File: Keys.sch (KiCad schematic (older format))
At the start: 24 parts

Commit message: experiment
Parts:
- SW? (x10): symbol Keys-rescue:SWITCH_PUSH-Keys-rescue-chgray-keyboard-rescue-chgray-keyboard-rescue -> Cherry-Symbols:SWITCH_PUSH
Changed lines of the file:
@@
 $EndDescr
 $Comp
-L Keys-rescue:SWITCH_PUSH-Keys-rescue-chgray-keyboard-rescue-chgray-keyboard-rescue SW?
+L Cherry-Symbols:SWITCH_PUSH SW?
 U 1 1 58964642
 P 2300 1600
@@
 KEY_ROW0
 $Comp
-L Keys-rescue:SWITCH_PUSH-Keys-rescue-chgray-keyboard-rescue-chgray-keyboard-rescue SW?
+L Cherry-Symbols:SWITCH_PUSH SW?
 U 1 1 589655C0
 P 3050 1600
@@
 $EndComp
 $Comp
-L Keys-rescue:SWITCH_PUSH-Keys-rescue-chgray-keyboard-rescue-chgray-keyboard-rescue SW?
+L Cherry-Symbols:SWITCH_PUSH SW?
 U 1 1 58965EBD
 P 2300 2300
@@
 	2700 1900 2700 2600
 $Comp
-L Keys-rescue:SWITCH_PUSH-Keys-rescue-chgray-keyboard-rescue-chgray-keyboard-rescue SW?
+L Cherry-Symbols:SWITCH_PUSH SW?
 U 1 1 603DF303
 P 3050 2300
@@
 	1800 2600 1800 3550
 $Comp
-L Keys-rescue:SWITCH_PUSH-Keys-rescue-chgray-keyboard-rescue-chgray-keyboard-rescue SW?
+L Cherry-Symbols:SWITCH_PUSH SW?
 U 1 1 603E8C3D
 P 2250 3250
@@
 	1800 3550 1800 4500
 $Comp
-L Keys-rescue:SWITCH_PUSH-Keys-rescue-chgray-keyboard-rescue-chgray-keyboard-rescue SW?
+L Cherry-Symbols:SWITCH_PUSH SW?
 U 1 1 6056C022
 P 2250 4200
@@
 Connection ~ 2700 3550
 $Comp
-L Keys-rescue:SWITCH_PUSH-Keys-rescue-chgray-keyboard-rescue-chgray-keyboard-rescue SW?
+L Cherry-Symbols:SWITCH_PUSH SW?
 U 1 1 60585067
 P 2250 5150
@@
 	2700 5450 2900 5450
 $Comp
-L Keys-rescue:SWITCH_PUSH-Keys-rescue-chgray-keyboard-rescue-chgray-keyboard-rescue SW?
+L Cherry-Symbols:SWITCH_PUSH SW?
 U 1 1 605950C9
 P 2250 6050
@@
 	1800 6350 2100 6350
 $Comp
-L Keys-rescue:SWITCH_PUSH-Keys-rescue-chgray-keyboard-rescue-chgray-keyboard-rescue SW?
+L Cherry-Symbols:SWITCH_PUSH SW?
 U 1 1 605950DC
 P 3050 6050
@@
 	3000 5450 3100 5450
 $Comp
-L Keys-rescue:SWITCH_PUSH-Keys-rescue-chgray-keyboard-rescue-chgray-keyboard-rescue SW?
+L Cherry-Symbols:SWITCH_PUSH SW?
 U 1 1 6058507A
 P 3050 5150

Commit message: experiment
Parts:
- D1, D10, D11, D12, D2, D3, D4, D5, D6, D7, D8, D9: renamed from D?; symbol Keys-rescue:D-Keys-rescue-chgray-keyboard-rescue-chgray-keyboard-rescue -> Cherry-Symbols:DIODE
- gave numbers to parts that had none: 12
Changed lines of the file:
@@
 $Descr A4 11693 8268
 encoding utf-8
-Sheet 1 1
+Sheet 1 2
 Title ""
 Date ""
@@
 $EndDescr
 $Comp
-L Cherry-Symbols:SWITCH_PUSH SW?
+L Cherry-Symbols:SWITCH_PUSH SW5
 U 1 1 58964642
 P 2300 1600
-F 0 "SW?" H 2450 1710 50  0000 C CNN
+F 0 "SW5" H 2450 1710 50  0000 C CNN
 F 1 "KEY_Q" H 2300 1520 50  0000 C CNN
 F 2 "CherryKeys:CHERRY_PCB_100H" H 2300 1600 60  0001 C CNN
@@
 $EndComp
 $Comp
-L Keys-rescue:D-Keys-rescue-chgray-keyboard-rescue-chgray-keyboard-rescue D?
+L Cherry-Symbols:DIODE D5
 U 1 1 5896466F
 P 2300 1900
-F 0 "D?" H 2300 2000 50  0000 C CNN
+F 0 "D5" H 2300 2000 50  0000 C CNN
 F 1 "D" H 2300 1800 50  0000 C CNN
 F 2 "Diode_SMD:D_0201_0603Metric" H 2300 1900 50  0001 C CNN
@@
 KEY_ROW0
 $Comp
-L Cherry-Symbols:SWITCH_PUSH SW?
+L Cherry-Symbols:SWITCH_PUSH SW7
 U 1 1 589655C0
 P 3050 1600
-F 0 "SW?" H 3200 1710 50  0000 C CNN
+F 0 "SW7" H 3200 1710 50  0000 C CNN
 F 1 "KEY_W" H 3050 1520 50  0000 C CNN
 F 2 "CherryKeys:CHERRY_PCB_100H" H 3050 1600 60  0000 C CNN
@@
 $EndComp
 $Comp
-L Keys-rescue:D-Keys-rescue-chgray-keyboard-rescue-chgray-keyboard-rescue D?
+L Cherry-Symbols:DIODE D7
 U 1 1 589655C6
 P 3050 1900
-F 0 "D?" H 3050 2000 50  0000 C CNN
+F 0 "D7" H 3050 2000 50  0000 C CNN
 F 1 "D" H 3050 1800 50  0000 C CNN
 F 2 "Diode_SMD:D_0201_0603Metric" H 3050 1900 50  0001 C CNN
@@
 $EndComp
 $Comp
-L Cherry-Symbols:SWITCH_PUSH SW?
+L Cherry-Symbols:SWITCH_PUSH SW6
 U 1 1 58965EBD
 P 2300 2300
-F 0 "SW?" H 2450 2410 50  0000 C CNN
+F 0 "SW6" H 2450 2410 50  0000 C CNN
 F 1 "KEY_A" H 2300 2220 50  0000 C CNN
 F 2 "CherryKeys:CHERRY_PCB_100H" H 2300 2300 60  0001 C CNN
@@
 $EndComp
 $Comp
-L Keys-rescue:D-Keys-rescue-chgray-keyboard-rescue-chgray-keyboard-rescue D?
+L Cherry-Symbols:DIODE D6
 U 1 1 58965EC3
 P 2300 2600
-F 0 "D?" H 2300 2700 50  0000 C CNN
+F 0 "D6" H 2300 2700 50  0000 C CNN
 F 1 "D" H 2300 2500 50  0000 C CNN
 F 2 "Diode_SMD:D_0201_0603Metric" H 2300 2600 50  0001 C CNN
@@
 	2700 1900 2700 2600
 $Comp
-L Cherry-Symbols:SWITCH_PUSH SW?
+L Cherry-Symbols:SWITCH_PUSH SW8
 U 1 1 603DF303
 P 3050 2300
-F 0 "SW?" H 3200 2410 50  0000 C CNN
+F 0 "SW8" H 3200 2410 50  0000 C CNN
 F 1 "KEY_W" H 3050 2220 50  0000 C CNN
 F 2 "CherryKeys:CHERRY_PCB_100H" H 3050 2300 60  0001 C CNN
@@
 	3000 1900 3100 1900
 $Comp
-L Keys-rescue:D-Keys-rescue-chgray-keyboard-rescue-chgray-keyboard-rescue D?
+L Cherry-Symbols:DIODE D8
 U 1 1 603E2BDF
 P 3050 2600
-F 0 "D?" H 3050 2700 50  0000 C CNN
+F 0 "D8" H 3050 2700 50  0000 C CNN
 F 1 "D" H 3050 2500 50  0000 C CNN
 F 2 "Diode_SMD:D_0201_0603Metric" H 3050 2600 50  0001 C CNN
@@
 	1800 2600 1800 3550
 $Comp
-L Cherry-Symbols:SWITCH_PUSH SW?
+L Cherry-Symbols:SWITCH_PUSH SW1
 U 1 1 603E8C3D
 P 2250 3250
-F 0 "SW?" H 2400 3360 50  0000 C CNN
+F 0 "SW1" H 2400 3360 50  0000 C CNN
 F 1 "KEY_W" H 2250 3170 50  0000 C CNN
 F 2 "CherryKeys:CHERRY_PCB_100H" H 2250 3250 60  0001 C CNN
@@
 $EndComp
 $Comp
-L Keys-rescue:D-Keys-rescue-chgray-keyboard-rescue-chgray-keyboard-rescue D?
+L Cherry-Symbols:DIODE D1
 U 1 1 603E8C43
 P 2250 3550
-F 0 "D?" H 2250 3650 50  0000 C CNN
+F 0 "D1" H 2250 3650 50  0000 C CNN
 F 1 "D" H 2250 3450 50  0000 C CNN
 F 2 "Diode_SMD:D_0201_0603Metric" H 2250 3550 50  0001 C CNN
@@
 	1800 3550 2100 3550
 $Comp
-L Cherry-Symbols:SWITCH_PUSH SW?
+L Cherry-Symbols:SWITCH_PUSH SW9
 U 1 1 603EBFA8
 P 3050 3250
-F 0 "SW?" H 3200 3360 50  0000 C CNN
+F 0 "SW9" H 3200 3360 50  0000 C CNN
 F 1 "KEY_W" H 3050 3170 50  0000 C CNN
 F 2 "CherryKeys:CHERRY_PCB_100H" H 3050 3250 60  0000 C CNN
@@
 	1800 3550 1800 4500
 $Comp
-L Cherry-Symbols:SWITCH_PUSH SW?
+L Cherry-Symbols:SWITCH_PUSH SW2
 U 1 1 6056C022
 P 2250 4200
-F 0 "SW?" H 2400 4310 50  0000 C CNN
+F 0 "SW2" H 2400 4310 50  0000 C CNN
 F 1 "KEY_W" H 2250 4120 50  0000 C CNN
 F 2 "CherryKeys:CHERRY_PCB_100H" H 2250 4200 60  0001 C CNN
@@
 $EndComp
 $Comp
-L Keys-rescue:D-Keys-rescue-chgray-keyboard-rescue-chgray-keyboard-rescue D?
+L Cherry-Symbols:DIODE D2
 U 1 1 6056C028
 P 2250 4500
-F 0 "D?" H 2250 4600 50  0000 C CNN
+F 0 "D2" H 2250 4600 50  0000 C CNN
 F 1 "D8" H 2250 4400 50  0000 C CNN
 F 2 "Diode_SMD:D_0201_0603Metric" H 2250 4500 50  0001 C CNN
@@
 	1800 4500 2100 4500
 $Comp
-L Cherry-Symbols:SWITCH_PUSH SW?
+L Cherry-Symbols:SWITCH_PUSH SW10
 U 1 1 6056C037
 P 3050 4200
-F 0 "SW?" H 3200 4310 50  0000 C CNN
+F 0 "SW10" H 3200 4310 50  0000 C CNN
 F 1 "KEY_W" H 3050 4120 50  0000 C CNN
 F 2 "CherryKeys:CHERRY_PCB_100H" H 3050 4200 60  0000 C CNN
@@
 $EndComp
 $Comp
-L Keys-rescue:D-Keys-rescue-chgray-keyboard-rescue-chgray-keyboard-rescue D?
+L Cherry-Symbols:DIODE D10
 U 1 1 6056C03D
 P 3050 4500
-F 0 "D?" H 3050 4600 50  0000 C CNN
+F 0 "D10" H 3050 4600 50  0000 C CNN
 F 1 "D9" H 3050 4400 50  0000 C CNN
 F 2 "Diode_SMD:D_0201_0603Metric" H 3050 4500 50  0001 C CNN
@@
 Connection ~ 2700 3550
 $Comp
-L Cherry-Symbols:SWITCH_PUSH SW?
+L Cherry-Symbols:SWITCH_PUSH SW3
 U 1 1 60585067
 P 2250 5150
-F 0 "SW?" H 2400 5260 50  0000 C CNN
+F 0 "SW3" H 2400 5260 50  0000 C CNN
 F 1 "KEY_W" H 2250 5070 50  0000 C CNN
 F 2 "CherryKeys:CHERRY_PCB_100H" H 2250 5150 60  0001 C CNN
@@
 $EndComp
 $Comp
-L Keys-rescue:D-Keys-rescue-chgray-keyboard-rescue-chgray-keyboard-rescue D?
+L Cherry-Symbols:DIODE D3
 U 1 1 6058506D
 P 2250 5450
-F 0 "D?" H 2250 5550 50  0000 C CNN
+F 0 "D3" H 2250 5550 50  0000 C CNN
 F 1 "D10" H 2250 5350 50  0000 C CNN
 F 2 "Diode_SMD:D_0201_0603Metric" H 2250 5450 50  0001 C CNN
@@
 	1800 5450 2100 5450
 $Comp
-L Keys-rescue:D-Keys-rescue-chgray-keyboard-rescue-chgray-keyboard-rescue D?
+L Cherry-Symbols:DIODE D11
 U 1 1 60585080
 P 3050 5450
-F 0 "D?" H 3050 5550 50  0000 C CNN
+F 0 "D11" H 3050 5550 50  0000 C CNN
 F 1 "D11" H 3050 5350 50  0000 C CNN
 F 2 "Diode_SMD:D_0201_0603Metric" H 3050 5450 50  0001 C CNN
@@
 	2700 5450 2900 5450
 $Comp
-L Cherry-Symbols:SWITCH_PUSH SW?
+L Cherry-Symbols:SWITCH_PUSH SW4
 U 1 1 605950C9
 P 2250 6050
-F 0 "SW?" H 2400 6160 50  0000 C CNN
+F 0 "SW4" H 2400 6160 50  0000 C CNN
 F 1 "KEY_W" H 2250 5970 50  0000 C CNN
 F 2 "CherryKeys:CHERRY_PCB_100H" H 2250 6050 60  0001 C CNN
@@
 $EndComp
 $Comp
-L Keys-rescue:D-Keys-rescue-chgray-keyboard-rescue-chgray-keyboard-rescue D?
+L Cherry-Symbols:DIODE D4
 U 1 1 605950CF
 P 2250 6350
-F 0 "D?" H 2250 6450 50  0000 C CNN
+F 0 "D4" H 2250 6450 50  0000 C CNN
 F 1 "D12" H 2250 6250 50  0000 C CNN
 F 2 "Diode_SMD:D_0201_0603Metric" H 2250 6350 50  0000 C CNN
@@
 	1800 6350 2100 6350
 $Comp
-L Cherry-Symbols:SWITCH_PUSH SW?
+L Cherry-Symbols:SWITCH_PUSH SW12
 U 1 1 605950DC
 P 3050 6050
-F 0 "SW?" H 3200 6160 50  0000 C CNN
+F 0 "SW12" H 3200 6160 50  0000 C CNN
 F 1 "KEY_W" H 3050 5970 50  0000 C CNN
 F 2 "CherryKeys:CHERRY_PCB_100H" H 3050 6050 60  0001 C CNN
@@
 $EndComp
 $Comp
-L Keys-rescue:D-Keys-rescue-chgray-keyboard-rescue-chgray-keyboard-rescue D?
+L Cherry-Symbols:DIODE D12
 U 1 1 605950E2
 P 3050 6350
-F 0 "D?" H 3050 6450 50  0000 C CNN
+F 0 "D12" H 3050 6450 50  0000 C CNN
 F 1 "D13" H 3050 6250 50  0000 C CNN
 F 2 "Diode_SMD:D_0201_0603Metric" H 3050 6350 50  0001 C CNN
@@
 	3000 5450 3100 5450
 $Comp
-L Cherry-Symbols:SWITCH_PUSH SW?
+L Cherry-Symbols:SWITCH_PUSH SW11
 U 1 1 6058507A
 P 3050 5150
-F 0 "SW?" H 3200 5260 50  0000 C CNN
+F 0 "SW11" H 3200 5260 50  0000 C CNN
 F 1 "KEY_W" H 3050 5070 50  0000 C CNN
 F 2 "CherryKeys:CHERRY_PCB_100H" H 3050 5150 60  0001 C CNN
@@
 $EndComp
 $Comp
-L Keys-rescue:D-Keys-rescue-chgray-keyboard-rescue-chgray-keyboard-rescue D?
+L Cherry-Symbols:DIODE D9
 U 1 1 603EBFAE
 P 3050 3550
-F 0 "D?" H 3050 3650 50  0000 C CNN
+F 0 "D9" H 3050 3650 50  0000 C CNN
 F 1 "D" H 3050 3450 50  0000 C CNN
 F 2 "Diode_SMD:D_0201_0603Metric" H 3050 3550 50  0001 C CNN

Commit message: working
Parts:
- D1, D10, D11, D12, D2, D3, D4, D5, D6, D7, D8, D9: symbol Cherry-Symbols:DIODE -> Cherry-Symbol:DIODE
- SW1, SW10, SW11, SW12, SW2, SW3, SW4, SW5, SW6, SW7, SW8, SW9: symbol Cherry-Symbols:SWITCH_PUSH -> Cherry-Symbol:SWITCH_PUSH
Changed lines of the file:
@@
 $Descr A4 11693 8268
 encoding utf-8
-Sheet 1 2
+Sheet 1 1
 Title ""
 Date ""
@@
 $EndDescr
 $Comp
-L Cherry-Symbols:SWITCH_PUSH SW5
+L Cherry-Symbol:SWITCH_PUSH SW5
 U 1 1 58964642
 P 2300 1600
 F 0 "SW5" H 2450 1710 50  0000 C CNN
 F 1 "KEY_Q" H 2300 1520 50  0000 C CNN
-F 2 "CherryKeys:CHERRY_PCB_100H" H 2300 1600 60  0001 C CNN
+F 2 "CherryKeys:CHERRY_PCB_100H" H 2300 1600 60  0000 C CNN
 F 3 "" H 2300 1600 60  0001 C CNN
 	1    2300 1600
@@
 $EndComp
 $Comp
-L Cherry-Symbols:DIODE D5
+L Cherry-Symbol:DIODE D5
 U 1 1 5896466F
 P 2300 1900
@@
 KEY_ROW0
 $Comp
-L Cherry-Symbols:SWITCH_PUSH SW7
+L Cherry-Symbol:SWITCH_PUSH SW7
 U 1 1 589655C0
 P 3050 1600
@@
 $EndComp
 $Comp
-L Cherry-Symbols:DIODE D7
+L Cherry-Symbol:DIODE D7
 U 1 1 589655C6
 P 3050 1900
@@
 $EndComp
 $Comp
-L Cherry-Symbols:SWITCH_PUSH SW6
+L Cherry-Symbol:SWITCH_PUSH SW6
 U 1 1 58965EBD
 P 2300 2300
@@
 $EndComp
 $Comp
-L Cherry-Symbols:DIODE D6
+L Cherry-Symbol:DIODE D6
 U 1 1 58965EC3
 P 2300 2600
@@
 	2700 1900 2700 2600
 $Comp
-L Cherry-Symbols:SWITCH_PUSH SW8
+L Cherry-Symbol:SWITCH_PUSH SW8
 U 1 1 603DF303
 P 3050 2300
@@
 	3000 1900 3100 1900
 $Comp
-L Cherry-Symbols:DIODE D8
+L Cherry-Symbol:DIODE D8
 U 1 1 603E2BDF
 P 3050 2600
@@
 	1800 2600 1800 3550
 $Comp
-L Cherry-Symbols:SWITCH_PUSH SW1
+L Cherry-Symbol:SWITCH_PUSH SW1
 U 1 1 603E8C3D
 P 2250 3250
@@
 $EndComp
 $Comp
-L Cherry-Symbols:DIODE D1
+L Cherry-Symbol:DIODE D1
 U 1 1 603E8C43
 P 2250 3550
@@
 	1800 3550 2100 3550
 $Comp
-L Cherry-Symbols:SWITCH_PUSH SW9
+L Cherry-Symbol:SWITCH_PUSH SW9
 U 1 1 603EBFA8
 P 3050 3250
@@
 	1800 3550 1800 4500
 $Comp
-L Cherry-Symbols:SWITCH_PUSH SW2
+L Cherry-Symbol:SWITCH_PUSH SW2
 U 1 1 6056C022
 P 2250 4200
@@
 $EndComp
 $Comp
-L Cherry-Symbols:DIODE D2
+L Cherry-Symbol:DIODE D2
 U 1 1 6056C028
 P 2250 4500
@@
 	1800 4500 2100 4500
 $Comp
-L Cherry-Symbols:SWITCH_PUSH SW10
+L Cherry-Symbol:SWITCH_PUSH SW10
 U 1 1 6056C037
 P 3050 4200
@@
 $EndComp
 $Comp
-L Cherry-Symbols:DIODE D10
+L Cherry-Symbol:DIODE D10
 U 1 1 6056C03D
 P 3050 4500
@@
 Connection ~ 2700 3550
 $Comp
-L Cherry-Symbols:SWITCH_PUSH SW3
+L Cherry-Symbol:SWITCH_PUSH SW3
 U 1 1 60585067
 P 2250 5150
@@
 $EndComp
 $Comp
-L Cherry-Symbols:DIODE D3
+L Cherry-Symbol:DIODE D3
 U 1 1 6058506D
 P 2250 5450
@@
 	1800 5450 2100 5450
 $Comp
-L Cherry-Symbols:DIODE D11
+L Cherry-Symbol:DIODE D11
 U 1 1 60585080
 P 3050 5450
@@
 	2700 5450 2900 5450
 $Comp
-L Cherry-Symbols:SWITCH_PUSH SW4
+L Cherry-Symbol:SWITCH_PUSH SW4
 U 1 1 605950C9
 P 2250 6050
@@
 $EndComp
 $Comp
-L Cherry-Symbols:DIODE D4
+L Cherry-Symbol:DIODE D4
 U 1 1 605950CF
 P 2250 6350
@@
 	1800 6350 2100 6350
 $Comp
-L Cherry-Symbols:SWITCH_PUSH SW12
+L Cherry-Symbol:SWITCH_PUSH SW12
 U 1 1 605950DC
 P 3050 6050
@@
 $EndComp
 $Comp
-L Cherry-Symbols:DIODE D12
+L Cherry-Symbol:DIODE D12
 U 1 1 605950E2
 P 3050 6350
@@
 	3000 5450 3100 5450
 $Comp
-L Cherry-Symbols:SWITCH_PUSH SW11
+L Cherry-Symbol:SWITCH_PUSH SW11
 U 1 1 6058507A
 P 3050 5150
@@
 $EndComp
 $Comp
-L Cherry-Symbols:DIODE D9
+L Cherry-Symbol:DIODE D9
 U 1 1 603EBFAE
 P 3050 3550

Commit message: experiment
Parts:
- D1, D5, D6, D7, D8, D9: value D -> DIODE; footprint Diode_SMD:D_0201_0603Metric -> CherryKeys:CHERRY_MX_DIODE
- D10: value D9 -> DIODE; footprint Diode_SMD:D_0201_0603Metric -> CherryKeys:CHERRY_MX_DIODE
- D11: value D11 -> DIODE; footprint Diode_SMD:D_0201_0603Metric -> CherryKeys:CHERRY_MX_DIODE
- D12: value D13 -> DIODE; footprint Diode_SMD:D_0201_0603Metric -> CherryKeys:CHERRY_MX_DIODE
- D2: value D8 -> DIODE; footprint Diode_SMD:D_0201_0603Metric -> CherryKeys:CHERRY_MX_DIODE
- D3: value D10 -> DIODE; footprint Diode_SMD:D_0201_0603Metric -> CherryKeys:CHERRY_MX_DIODE
- D4: value D12 -> DIODE; footprint Diode_SMD:D_0201_0603Metric -> CherryKeys:CHERRY_MX_DIODE
- SW5: value KEY_Q -> KEY_W
- SW6: value KEY_A -> KEY_W
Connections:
- wire segments 84 -> 62

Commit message: working
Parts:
- added D13, D14, D15, D16, D17, D18, D19, D20, D21, D22, D23, D24, D25, D26, D27, D28, D29, D30, D31, D32, D33, D34, D35, D36, D37, D38, D39, D40, D41, D42, D43, D44, D45, D46, D47, D48, D49, D50, D51, D52, D53, D54, D55, D56, D57, D58, D59, D60: DIODE, CherryKeys:CHERRY_MX_DIODE, symbol chgray-keyboard-rescue:DIODE-Cherry-Symbol
- added SW13, SW14, SW15, SW16, SW17, SW18, SW19, SW20, SW21, SW22, SW23, SW24, SW25, SW26, SW27, SW28, SW29, SW30, SW31, SW32, SW33, SW34, SW35, SW36, SW37, SW38, SW39, SW40, SW41, SW42, SW43, SW44, SW45, SW46, SW47, SW48, SW49, SW50, SW51, SW52, SW53, SW54, SW55, SW56, SW57, SW58, SW59, SW60: KEY_W, CherryKeys:CHERRY_PCB_100H, symbol chgray-keyboard-rescue:SWITCH_PUSH-Cherry-Symbol
- D1, D10, D11, D12, D2, D3, D4, D5, D6, D7, D8, D9: symbol Cherry-Symbol:DIODE -> chgray-keyboard-rescue:DIODE-Cherry-Symbol
- SW1, SW10, SW11, SW12, SW2, SW3, SW4, SW5, SW6, SW7, SW8, SW9: symbol Cherry-Symbol:SWITCH_PUSH -> chgray-keyboard-rescue:SWITCH_PUSH-Cherry-Symbol
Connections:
- net labels added: KEY_COL2, KEY_COL3, KEY_COL4, KEY_COL5, KEY_COL6, KEY_COL7, KEY_COL8, KEY_COL9
- wire segments 62 -> 310

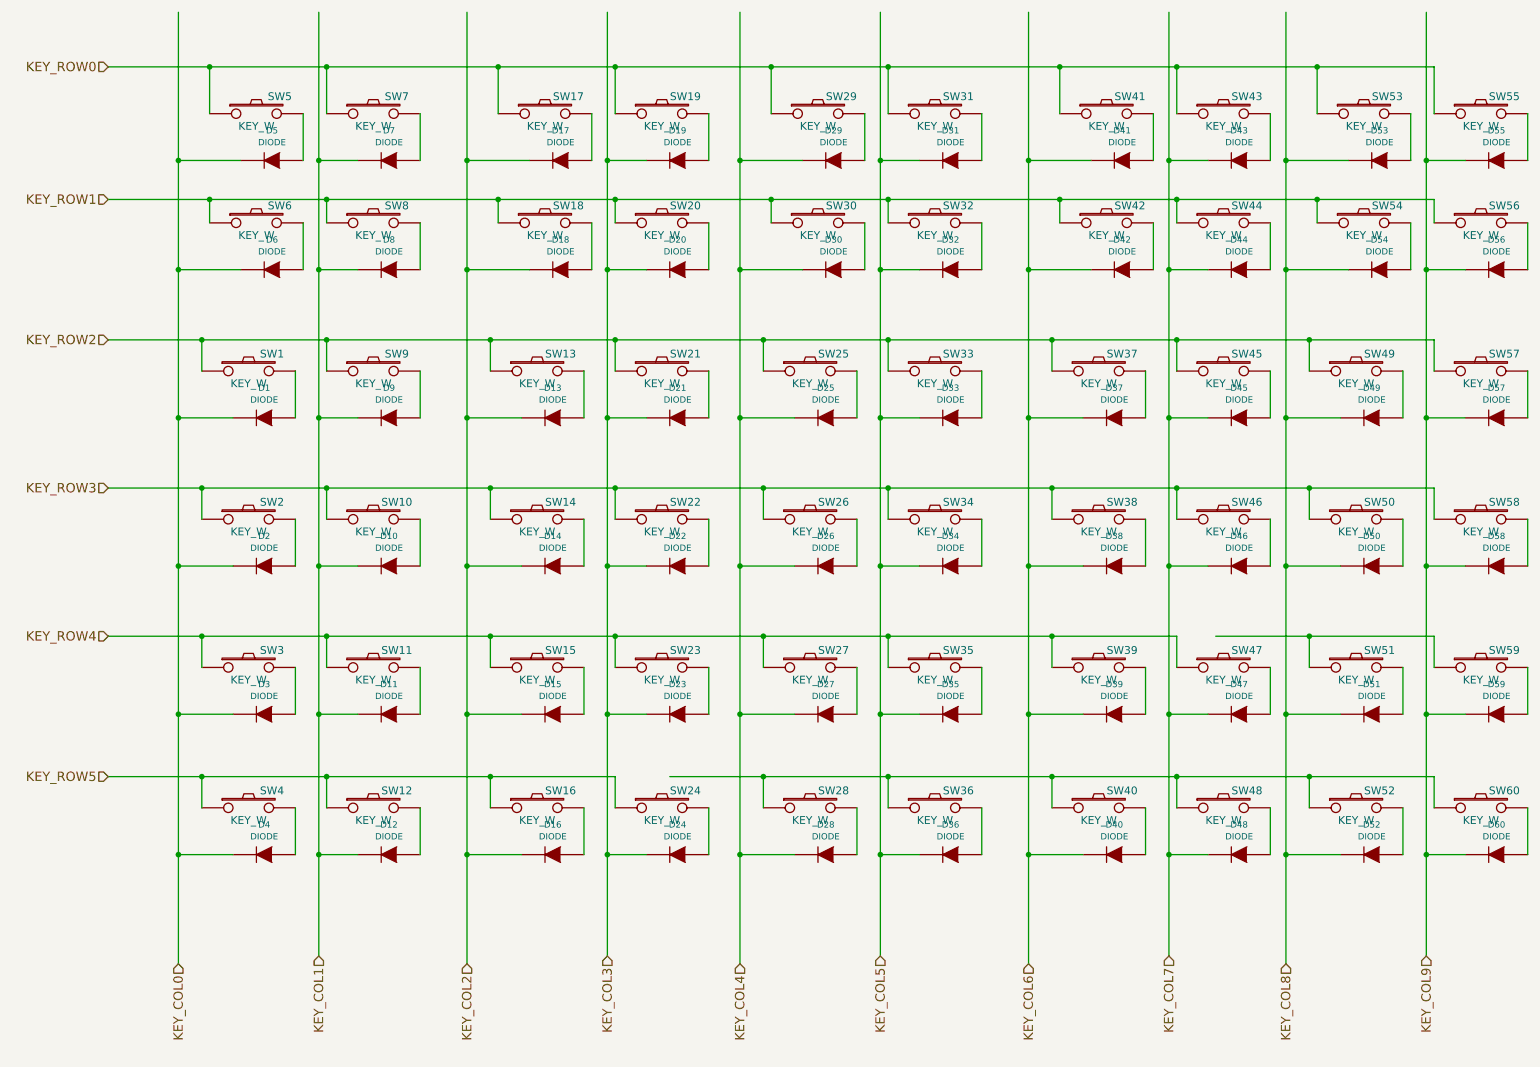
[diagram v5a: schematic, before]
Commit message: print as sent for pcb:1
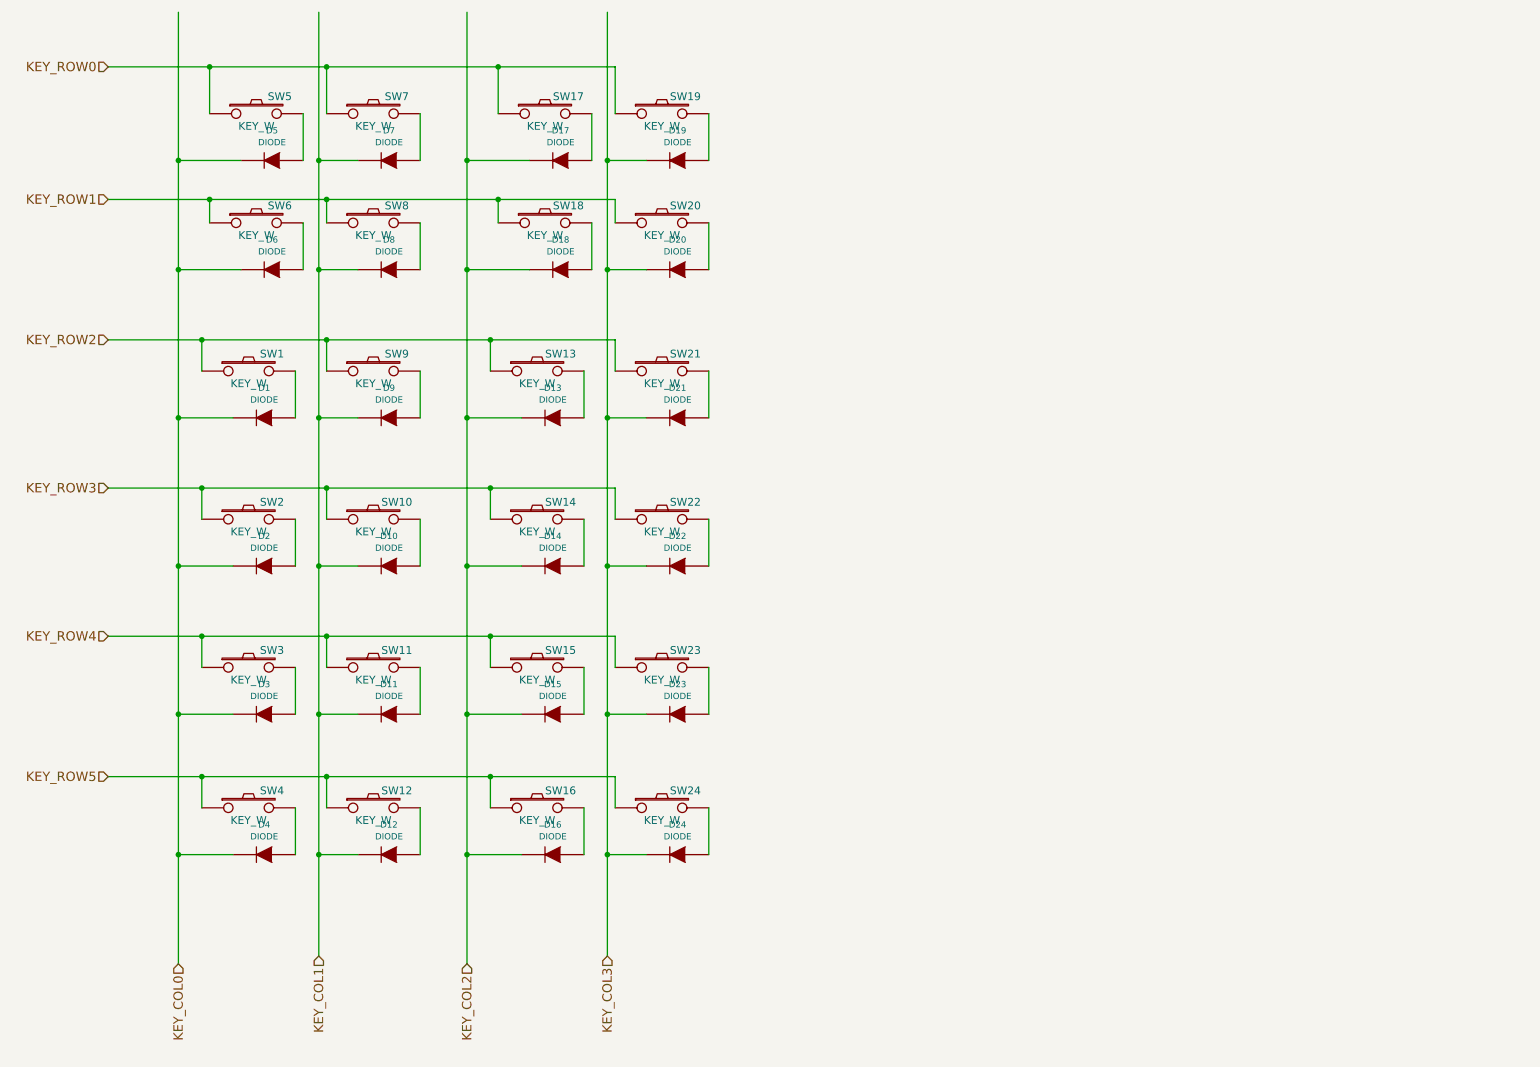
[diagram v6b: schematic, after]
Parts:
- removed D25, D26, D27, D28, D29, D30, D31, D32, D33, D34, D35, D36, D37, D38, D39, D40, D41, D42, D43, D44, D45, D46, D47, D48, D49, D50, D51, D52, D53, D54, D55, D56, D57, D58, D59, D60: DIODE, CherryKeys:CHERRY_MX_DIODE, symbol chgray-keyboard-rescue:DIODE-Cherry-Symbol
- removed SW25, SW26, SW27, SW28, SW29, SW30, SW31, SW32, SW33, SW34, SW35, SW36, SW37, SW38, SW39, SW40, SW41, SW42, SW43, SW44, SW45, SW46, SW47, SW48, SW49, SW50, SW51, SW52, SW53, SW54, SW55, SW56, SW57, SW58, SW59, SW60: KEY_W, CherryKeys:CHERRY_PCB_100H, symbol chgray-keyboard-rescue:SWITCH_PUSH-Cherry-Symbol
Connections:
- net labels removed: KEY_COL4, KEY_COL5, KEY_COL6, KEY_COL7, KEY_COL8, KEY_COL9
- wire segments 310 -> 124
